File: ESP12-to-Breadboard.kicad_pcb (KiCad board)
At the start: 2 copper layers, 22.9 x 20.1 mm, 3 parts, among them J1 Conn_01x08, J2 Conn_01x08, U1 ESP-12E

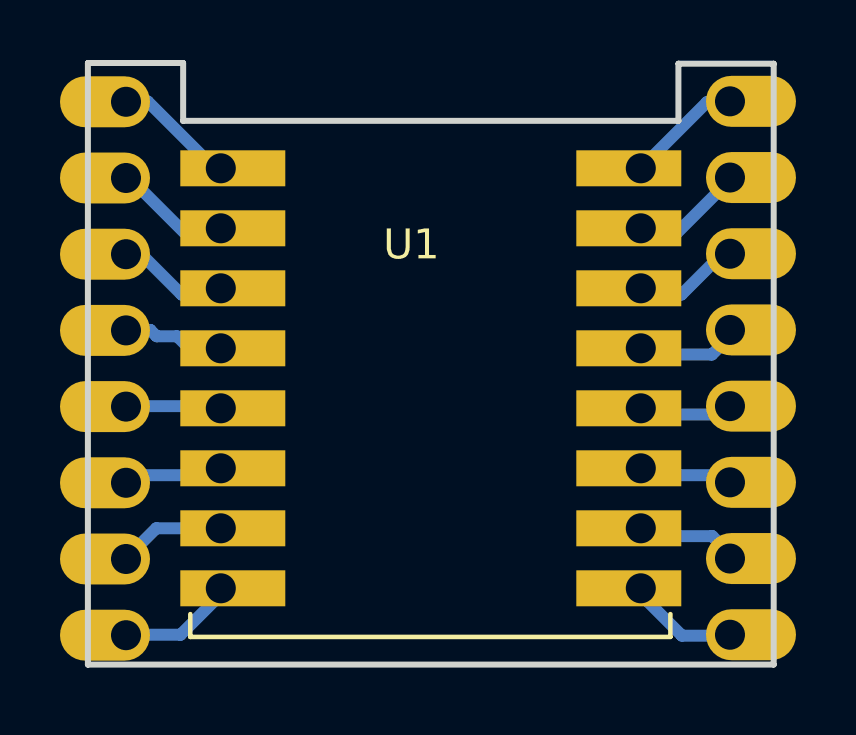
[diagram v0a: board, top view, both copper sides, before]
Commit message: Prepare for plotting
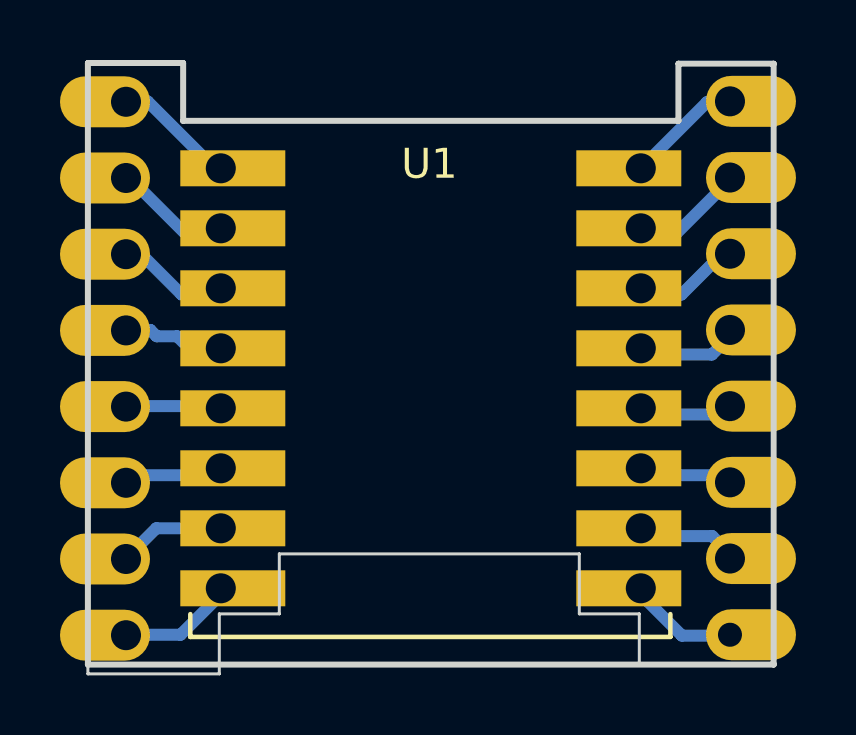
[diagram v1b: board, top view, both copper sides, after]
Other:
- board size 22.9 x 20.1 mm -> 22.9 x 20.4 mm
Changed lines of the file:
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@@
     (pad_to_mask_clearance 0)
     (pcbplotparams
-      (layerselection 0x00010fc_ffffffff)
+      (layerselection 0x0000000_fffffffe)
       (disableapertmacros false)
       (usegerberextensions false)
@@
       (hpglpendiameter 15.000000)
       (dxfpolygonmode true)
-      (dxfimperialunits true)
+      (dxfimperialunits false)
       (dxfusepcbnewfont true)
       (psnegative false)
@@
       (sketchpadsonfab false)
       (subtractmaskfromsilk false)
-      (outputformat 1)
+      (outputformat 3)
       (mirror false)
-      (drillshape 1)
+      (drillshape 0)
       (scaleselection 1)
-      (outputdirectory "")
+      (outputdirectory "plot")
     )
   )
@@
     (property "Sheetname" "")
     (attr through_hole)
-    (fp_text reference "U1" (at 6.35 2.54) (layer "F.SilkS")
+    (fp_text reference "U1" (at 6.95 -0.147) (layer "F.SilkS")
       (effects (font (size 1 1) (thickness 0.15)))
     )
@@
     (fp_line (start 1.27 -19.05) (end -1.27 -19.05) (layer "B.Fab") (width 0.1))
     (fp_line (start -1.27 0.635) (end -0.635 1.27) (layer "B.Fab") (width 0.1))
-    (pad "1" thru_hole oval (at 0 0) (size 3 1.7) (drill 1 (offset 0.7 0)) (layers *.Cu *.Mask)
+    (pad "1" thru_hole oval (at 0 0) (size 3 1.7) (drill 0.8 (offset 0.7 0)) (layers *.Cu *.Mask)
       (net 16 "Net-(J2-Pad1)") (pinfunction "Pin_1") (pintype "passive"))
     (pad "2" thru_hole oval (at 0 -2.54) (size 3 1.7) (drill 1 (offset 0.7 0)) (layers *.Cu *.Mask)
@@
   (gr_poly
     (pts
+      (xy 137.794998 75.565)
+      (xy 154.304998 75.565)
+      (xy 154.304998 73.66)
+      (xy 157.479998 73.66)
+      (xy 157.479998 93.689919)
+      (xy 153 93.689919)
+      (xy 153 92)
+      (xy 151 92)
+      (xy 151 90)
+      (xy 141 90)
+      (xy 141 92)
+      (xy 139 92)
+      (xy 139 94)
+      (xy 134.619999 94)
+      (xy 134.619999 73.63693)
+      (xy 137.794998 73.63693)
+    ) (layer "Edge.Cuts") (width 0.1) (fill none))
+  (gr_poly
+    (pts
